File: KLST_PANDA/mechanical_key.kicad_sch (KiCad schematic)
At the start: 4 parts, among them SW5 BUTTON

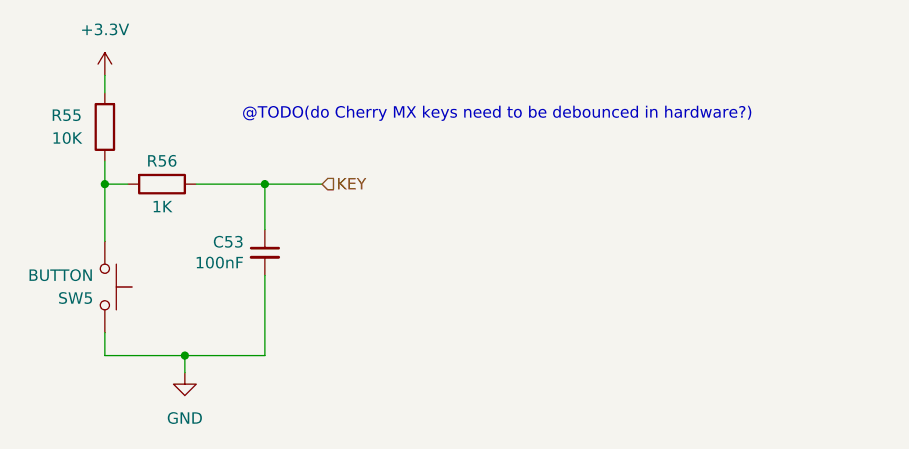
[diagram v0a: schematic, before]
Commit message: cleaned up
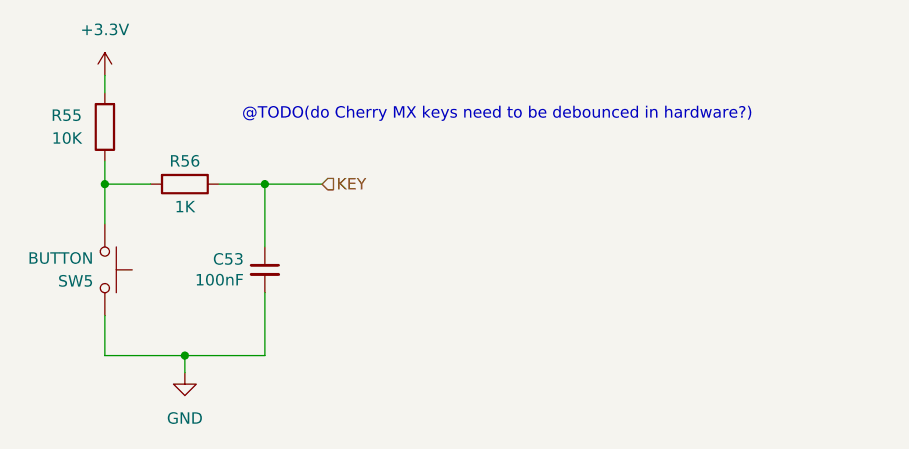
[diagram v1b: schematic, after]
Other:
- moved on the sheet: C53, R56, SW5
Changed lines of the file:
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@@
     (stroke (width 0) (type default))
   )
-  (wire (pts (xy 151.765 95.885) (xy 151.765 100.965))
-    (stroke (width 0) (type default))
-  )
-  (wire (pts (xy 151.765 106.045) (xy 151.765 114.935))
+  (wire (pts (xy 151.765 95.885) (xy 151.765 102.87))
+    (stroke (width 0) (type default))
+  )
+  (wire (pts (xy 151.765 107.95) (xy 151.765 114.935))
     (stroke (width 0) (type default))
   )
@@
     (stroke (width 0) (type default))
   )
-  (wire (pts (xy 144.145 95.885) (xy 151.765 95.885))
-    (stroke (width 0) (type default))
-  )
-  (wire (pts (xy 133.985 95.885) (xy 133.985 102.235))
-    (stroke (width 0) (type default))
-  )
-  (wire (pts (xy 133.985 114.935) (xy 133.985 112.395))
-    (stroke (width 0) (type default))
-  )
-  (wire (pts (xy 136.525 95.885) (xy 133.985 95.885))
+  (wire (pts (xy 146.685 95.885) (xy 151.765 95.885))
+    (stroke (width 0) (type default))
+  )
+  (wire (pts (xy 133.985 95.885) (xy 133.985 100.33))
+    (stroke (width 0) (type default))
+  )
+  (wire (pts (xy 133.985 114.935) (xy 133.985 110.49))
+    (stroke (width 0) (type default))
+  )
+  (wire (pts (xy 139.065 95.885) (xy 133.985 95.885))
     (stroke (width 0) (type default))
   )
@@
     )
   )
-  (symbol (lib_id "Switch:SW_Push") (at 133.985 107.315 270) (unit 1)
-    (in_bom yes) (on_board yes) (dnp no)
-    (property "Reference" "SW5" (at 132.715 108.585 90)
+  (symbol (lib_id "Switch:SW_Push") (at 133.985 105.41 270) (unit 1)
+    (in_bom yes) (on_board yes) (dnp no)
+    (property "Reference" "SW5" (at 132.715 106.68 90)
       (effects (font (size 1.27 1.27)) (justify right))
     )
-    (property "Value" "BUTTON" (at 132.715 106.045 90)
+    (property "Value" "BUTTON" (at 132.715 104.14 90)
       (effects (font (size 1.27 1.27)) (justify right))
     )
-    (property "Footprint" "Cherry_MX:SW_Cherry_MX_PCB" (at 139.065 107.315 0)
-      (effects (font (size 1.27 1.27)) hide)
-    )
-    (property "Datasheet" "~" (at 139.065 107.315 0)
+    (property "Footprint" "Cherry_MX:SW_Cherry_MX_PCB" (at 139.065 105.41 0)
+      (effects (font (size 1.27 1.27)) hide)
+    )
+    (property "Datasheet" "~" (at 139.065 105.41 0)
       (effects (font (size 1.27 1.27)) hide)
     )
@@
     )
   )
-  (symbol (lib_id "Device:C_Small") (at 151.765 103.505 0) (mirror y) (unit 1)
-    (in_bom yes) (on_board yes) (dnp no)
-    (property "Reference" "C53" (at 149.4282 102.3366 0)
-      (effects (font (size 1.27 1.27)) (justify left))
-    )
-    (property "Value" "100nF" (at 149.4282 104.648 0)
-      (effects (font (size 1.27 1.27)) (justify left))
-    )
-    (property "Footprint" "Capacitor_SMD:C_0402_1005Metric" (at 151.765 103.505 0)
-      (effects (font (size 1.27 1.27)) hide)
-    )
-    (property "Datasheet" "~" (at 151.765 103.505 0)
-      (effects (font (size 1.27 1.27)) hide)
-    )
-    (property "MFR.Part #" "CL05B104KO5NNNC" (at 151.765 103.505 0)
-      (effects (font (size 1.27 1.27)) hide)
-    )
-    (property "LCSC Part #" "" (at 151.765 103.505 0)
-      (effects (font (size 1.27 1.27)) hide)
-    )
-    (property "Extended Part" "-" (at 151.765 103.505 0)
-      (effects (font (size 1.27 1.27)) hide)
-    )
-    (property "JLCPCB Part #" "C1525" (at 151.765 103.505 0)
+  (symbol (lib_id "Device:C_Small") (at 151.765 105.41 0) (mirror y) (unit 1)
+    (in_bom yes) (on_board yes) (dnp no)
+    (property "Reference" "C53" (at 149.4282 104.2416 0)
+      (effects (font (size 1.27 1.27)) (justify left))
+    )
+    (property "Value" "100nF" (at 149.4282 106.553 0)
+      (effects (font (size 1.27 1.27)) (justify left))
+    )
+    (property "Footprint" "Capacitor_SMD:C_0402_1005Metric" (at 151.765 105.41 0)
+      (effects (font (size 1.27 1.27)) hide)
+    )
+    (property "Datasheet" "~" (at 151.765 105.41 0)
+      (effects (font (size 1.27 1.27)) hide)
+    )
+    (property "MFR.Part #" "CL05B104KO5NNNC" (at 151.765 105.41 0)
+      (effects (font (size 1.27 1.27)) hide)
+    )
+    (property "LCSC Part #" "" (at 151.765 105.41 0)
+      (effects (font (size 1.27 1.27)) hide)
+    )
+    (property "Extended Part" "-" (at 151.765 105.41 0)
+      (effects (font (size 1.27 1.27)) hide)
+    )
+    (property "JLCPCB Part #" "C1525" (at 151.765 105.41 0)
       (effects (font (size 1.27 1.27)) hide)
     )
@@
     )
   )
-  (symbol (lib_id "Device:R") (at 140.335 95.885 270) (unit 1)
-    (in_bom yes) (on_board yes) (dnp no)
-    (property "Reference" "R56" (at 140.335 93.345 90)
-      (effects (font (size 1.27 1.27)))
-    )
-    (property "Value" "1K" (at 140.335 98.425 90)
-      (effects (font (size 1.27 1.27)))
-    )
-    (property "Footprint" "Resistor_SMD:R_0402_1005Metric" (at 140.335 94.107 90)
-      (effects (font (size 1.27 1.27)) hide)
-    )
-    (property "Datasheet" "~" (at 140.335 95.885 0)
-      (effects (font (size 1.27 1.27)) hide)
-    )
-    (property "MFR.Part #" "0402WGF1001TCE" (at 140.335 95.885 90)
-      (effects (font (size 1.27 1.27)) hide)
-    )
-    (property "LCSC Part #" "" (at 140.335 95.885 0)
-      (effects (font (size 1.27 1.27)) hide)
-    )
-    (property "Extended Part" "-" (at 140.335 95.885 0)
-      (effects (font (size 1.27 1.27)) hide)
-    )
-    (property "JLCPCB Part #" "C11702" (at 140.335 95.885 0)
-      (effects (font (size 1.27 1.27)) hide)
-    )
+  (symbol (lib_id "Device:R") (at 142.875 95.885 270) (unit 1)
+    (in_bom yes) (on_board yes) (dnp no)
+    (property "Reference" "R56" (at 142.875 93.345 90)
+      (effects (font (size 1.27 1.27)))
+    )
+    (property "Value" "1K" (at 142.875 98.425 90)
+      (effects (font (size 1.27 1.27)))
+    )
+    (property "Footprint" "Resistor_SMD:R_0402_1005Metric" (at 142.875 94.107 90)
+      (effects (font (size 1.27 1.27)) hide)
+    )
+    (property "Datasheet" "~" (at 142.875 95.885 0)
+      (effects (font (size 1.27 1.27)) hide)
+    )
+    (property "MFR.Part #" "0402WGF1001TCE" (at 142.875 95.885 90)
+      (effects (font (size 1.27 1.27)) hide)
+    )
+    (property "LCSC Part #" "" (at 142.875 95.885 0)
+      (effects (font (size 1.27 1.27)) hide)
+    )
+    (property "Extended Part" "-" (at 142.875 95.885 0)
+      (effects (font (size 1.27 1.27)) hide)
+    )
+    (property "JLCPCB Part #" "C11702" (at 142.875 95.885 0)
+      (effects (font (size 1.27 1.27)) hide)
+    )
